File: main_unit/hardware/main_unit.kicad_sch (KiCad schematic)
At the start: 14 parts, among them SW1 PTS636SM43SMTR LFS, U1 STM32H753ZIT6, Y1 ABM8G-25.000MHZ-18-D2Y-T, Y2 SC32S-7PF20PPM

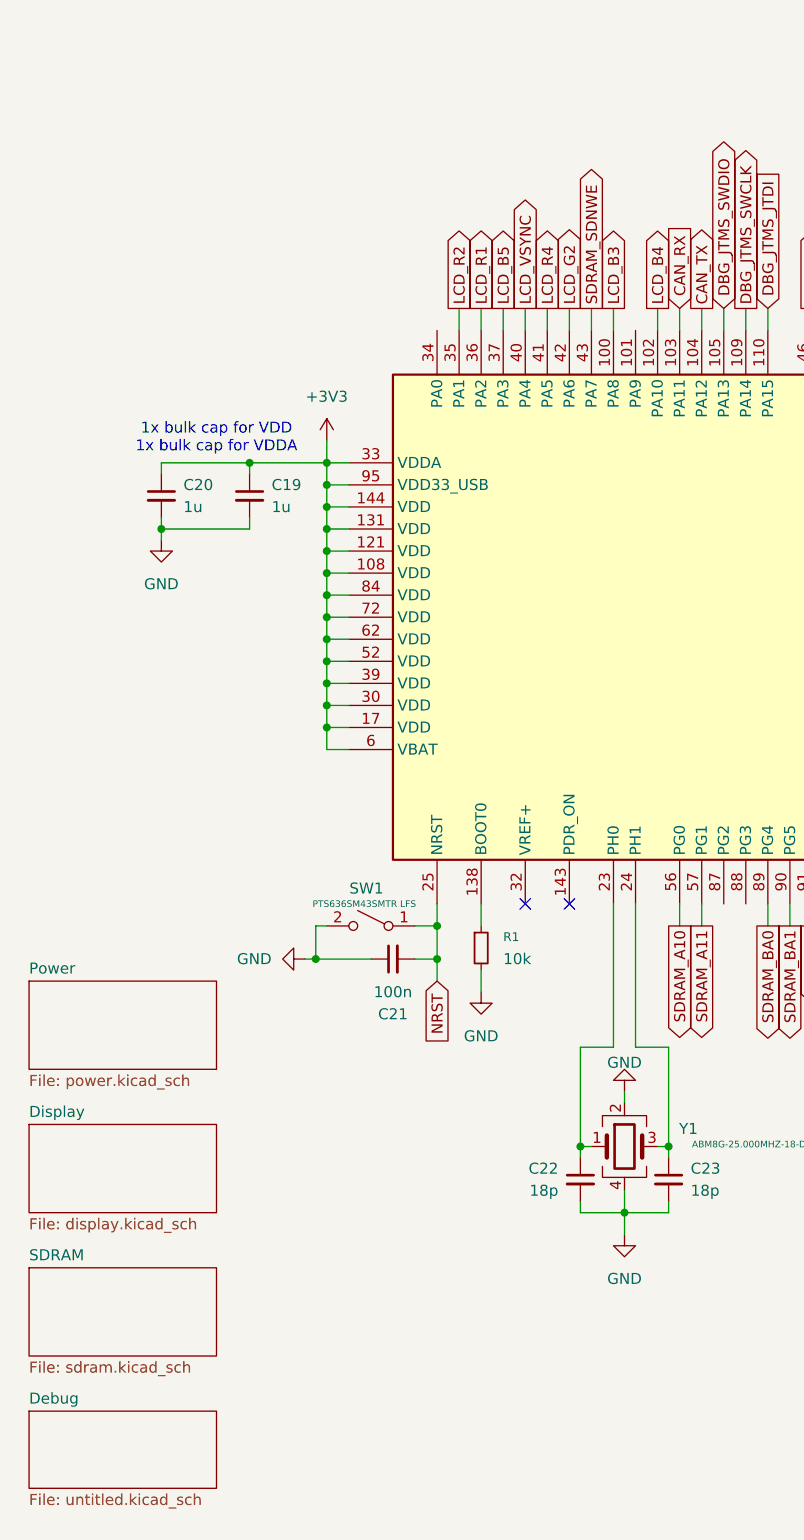
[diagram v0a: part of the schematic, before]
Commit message: main_unit/hardware: Rearrange more components, add CAN transceiver
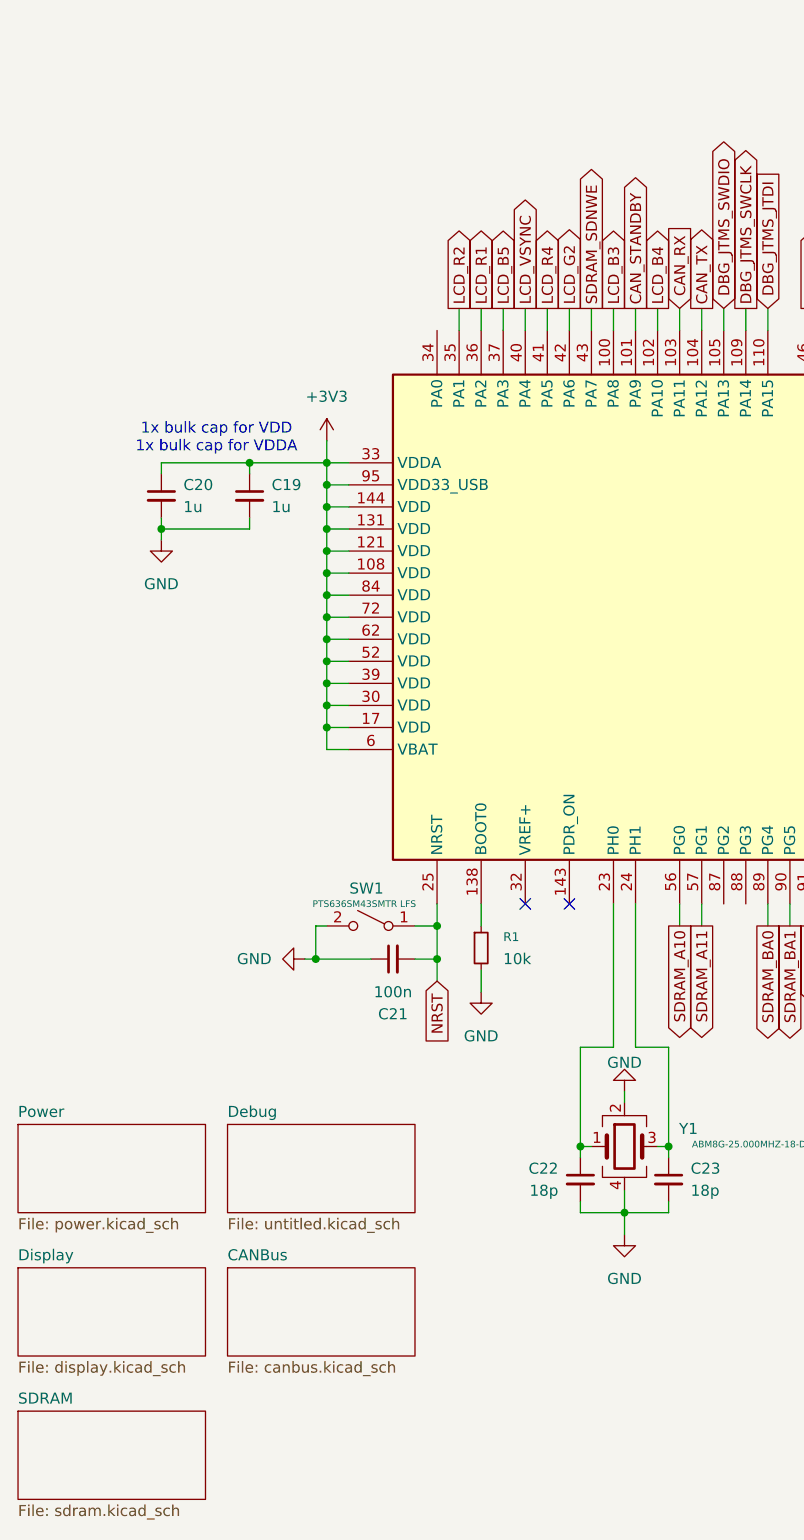
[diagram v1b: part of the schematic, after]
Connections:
- net CAN_STANDBY: now reaches U1.101 (PA9)
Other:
- added sheet CANBus (canbus.kicad_sch)
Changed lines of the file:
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@@
 	(wire
 		(pts
+			(xy 85.09 57.15) (xy 85.09 59.69)
+		)
+		(stroke
+			(width 0)
+			(type default)
+		)
+	)
+	(wire
+		(pts
 			(xy 168.91 57.15) (xy 168.91 59.69)
 		)
@@
 		)
 	)
+	(global_label "CAN_STANDBY"
+		(shape output)
+		(at 85.09 57.15 90)
+		(fields_autoplaced yes)
+		(effects
+			(font
+				(size 1.27 1.27)
+			)
+			(justify left)
+		)
+		(property "Intersheetrefs" "${INTERSHEET_REFS}"
+			(at 85.09 41.2833 90)
+			(effects
+				(font
+					(size 1.27 1.27)
+				)
+				(justify left)
+				(hide yes)
+			)
+		)
+	)
 	(global_label "SDRAM_D0"
 		(shape bidirectional)
@@
 	)
 	(sheet
-		(at 15.24 184.15)
-		(size 21.59 8.89)
+		(at 38.1 151.13)
+		(size 21.59 10.16)
 		(exclude_from_sim no)
 		(in_bom yes)
@@
 		)
 		(property "Sheetname" "Debug"
-			(at 15.24 183.4384 0)
+			(at 38.1 150.4184 0)
 			(effects
 				(font
@@
 		)
 		(property "Sheetfile" "untitled.kicad_sch"
-			(at 15.24 193.6246 0)
+			(at 38.1 161.8746 0)
 			(effects
 				(font
@@
 	)
 	(sheet
-		(at 15.24 167.64)
+		(at 38.1 167.64)
+		(size 21.59 10.16)
+		(exclude_from_sim no)
+		(in_bom yes)
+		(on_board yes)
+		(dnp no)
+		(fields_autoplaced yes)
+		(stroke
+			(width 0.1524)
+			(type solid)
+		)
+		(fill
+			(color 0 0 0 0.0000)
+		)
+		(property "Sheetname" "CANBus"
+			(at 38.1 166.9284 0)
+			(effects
+				(font
+					(size 1.27 1.27)
+				)
+				(justify left bottom)
+			)
+		)
+		(property "Sheetfile" "canbus.kicad_sch"
+			(at 38.1 178.3846 0)
+			(effects
+				(font
+					(size 1.27 1.27)
+				)
+				(justify left top)
+			)
+		)
+		(instances
+			(project "main_unit"
+				(path "/c1e2a568-b99f-4357-b0bb-65969671b711"
+					(page "6")
+				)
+			)
+		)
+	)
+	(sheet
+		(at 13.97 184.15)
 		(size 21.59 10.16)
 		(exclude_from_sim no)
@@
 		)
 		(property "Sheetname" "SDRAM"
-			(at 15.24 166.9284 0)
+			(at 13.97 183.4384 0)
 			(effects
 				(font
@@
 		)
 		(property "Sheetfile" "sdram.kicad_sch"
-			(at 15.24 178.3846 0)
+			(at 13.97 194.8946 0)
 			(effects
 				(font
@@
 	)
 	(sheet
-		(at 15.24 134.62)
+		(at 13.97 151.13)
 		(size 21.59 10.16)
 		(exclude_from_sim no)
@@
 		)
 		(property "Sheetname" "Power"
-			(at 15.24 133.9084 0)
+			(at 13.97 150.4184 0)
 			(effects
 				(font
@@
 		)
 		(property "Sheetfile" "power.kicad_sch"
-			(at 15.24 145.3646 0)
+			(at 13.97 161.8746 0)
 			(effects
 				(font
@@
 	)
 	(sheet
-		(at 15.24 151.13)
+		(at 13.97 167.64)
 		(size 21.59 10.16)
 		(exclude_from_sim no)
@@
 		)
 		(property "Sheetname" "Display"
-			(at 15.24 150.4184 0)
+			(at 13.97 166.9284 0)
 			(effects
 				(font
@@
 		)
 		(property "Sheetfile" "display.kicad_sch"
-			(at 15.24 161.8746 0)
+			(at 13.97 178.3846 0)
 			(effects
 				(font
@@
 		)
 		(property "Field2" ""
-			(at 15.24 151.13 0)
+			(at 13.97 167.64 0)
 			(effects
 				(font
